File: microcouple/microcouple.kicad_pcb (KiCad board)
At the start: 4 copper layers, 29.3 x 37.5 mm, 127 parts, among them J1 Conn_ARM_SWD_TagConnect_TC203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, P1 USB_C_Plug, Q1 AO3415, SW1 ~{RESET}, SW2 SW_SPDT_MSK12CO2, SW3 CS2, SW4 CS3, SW5 CS4, U1 USBLC6-2SC6, U2 RP2040, U3 MCP73831-2-OT, U4 LM3671MFX, U5 IRM-V838M3-C/TR1, U6 IS31FL3729, U7 CAP1188, X1 12MHz 12pF

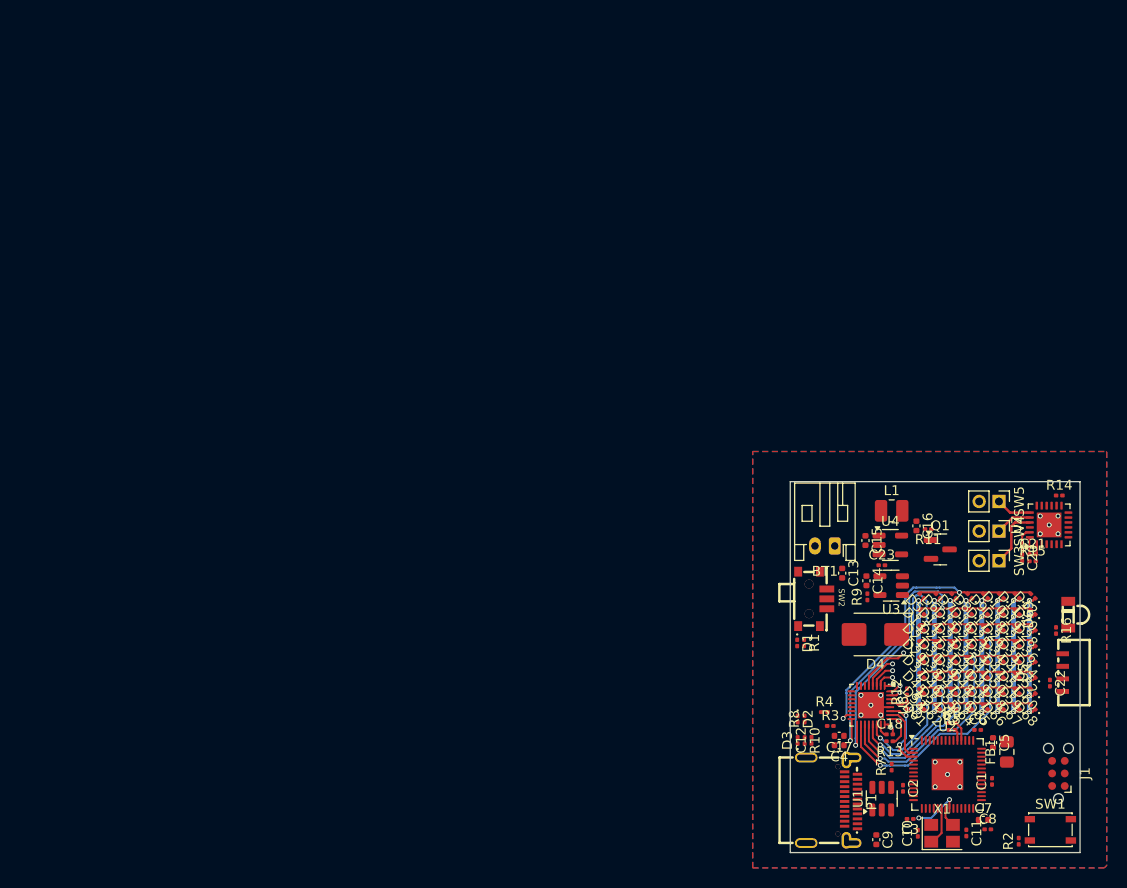
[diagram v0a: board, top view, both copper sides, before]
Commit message: Draft layout
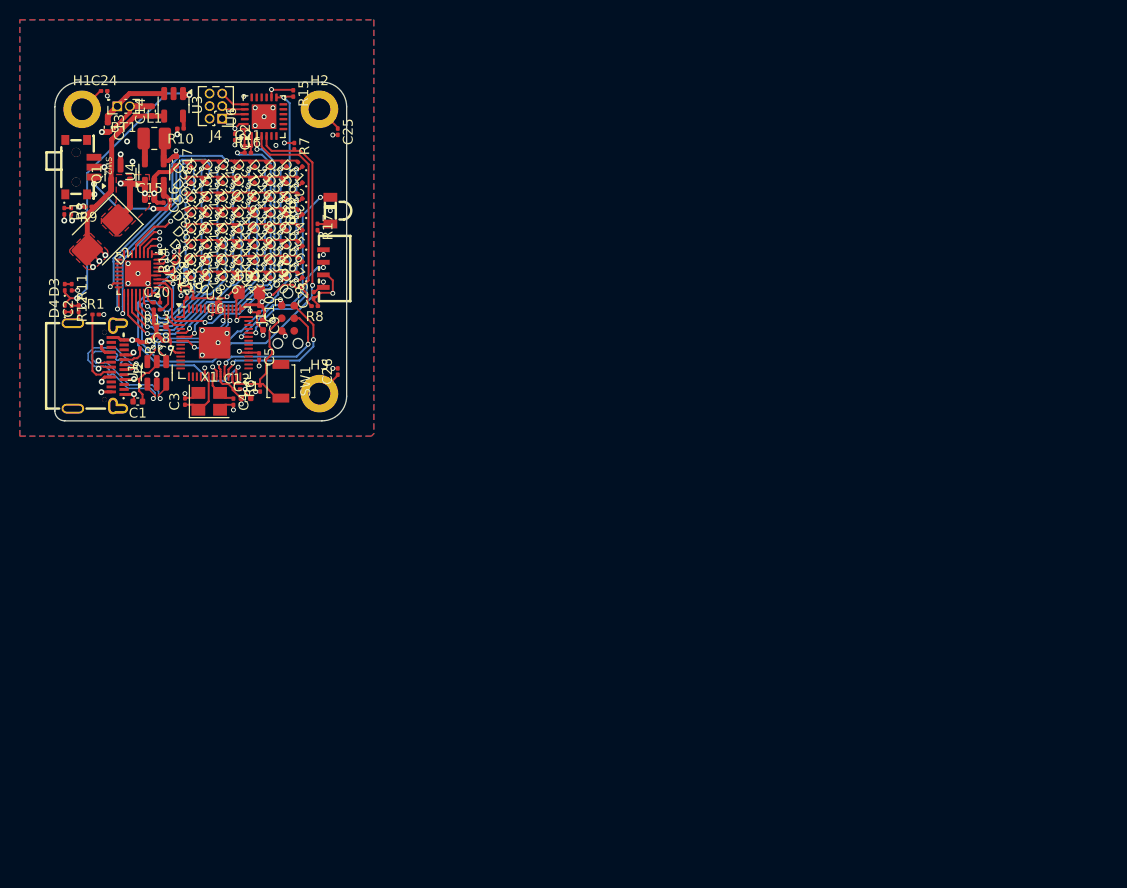
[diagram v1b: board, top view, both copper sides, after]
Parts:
- removed the C17 at (165.4, 110.7)
- removed the C9 at (169.2, 121.2)
- removed R5: 27R, Resistor_SMD:R_0201_0603Metric
- removed the R6 at (176.8, 109.4)
- removed SW3: CS2, Connector_PinHeader_2.00mm:PinHeader_1x02_P2.00mm_Vertical
- removed SW4: CS3, Connector_PinHeader_2.00mm:PinHeader_1x02_P2.00mm_Vertical
- removed SW5: CS4, Connector_PinHeader_2.00mm:PinHeader_1x02_P2.00mm_Vertical
- added C1: 4.7uF, Capacitor_SMD:C_0402_1005Metric, F.Cu at (94.5, 76.9)
- added C19: 100nF, Capacitor_SMD:C_0201_0603Metric, F.Cu at (99.8, 66.5)
- added C24: 100nF, Capacitor_SMD:C_0201_0603Metric, F.Cu at (91.1, 45.5)
- added C25: 100nF, Capacitor_SMD:C_0201_0603Metric, F.Cu at (114.8, 49.6)
- added C26: 100nF, Capacitor_SMD:C_0201_0603Metric, F.Cu at (114.8, 73.9)
- added H1: MountingHole_Pad, MountingHole:MountingHole_2.2mm_M2_DIN965_Pad, F.Cu at (88.9, 47.4)
- added H2: MountingHole_Pad, MountingHole:MountingHole_2.2mm_M2_DIN965_Pad, F.Cu at (112.9, 47.4)
- added H3: MountingHole_Pad, MountingHole:MountingHole_2.2mm_M2_DIN965_Pad, F.Cu at (112.9, 76.1)
- added J4: Conn_02x03_Odd_Even, Connector_PinHeader_1.27mm:PinHeader_2x03_P1.27mm_Vertical, F.Cu at (103.1, 48.3)
- added R2: 5.1k, Resistor_SMD:R_0201_0603Metric, F.Cu at (94.8, 71.2)
- BT1: footprint Connector_JST:JST_PH_S2B-PH-K_1x02_P2.00mm_Horizontal -> Connector_PinSocket_1.27mm:PinSocket_2x01_P1.27mm_Vertical
- J2: renamed from P1; value USB_C_Plug -> USB_C_Socket
- SW1: footprint Button_Switch_SMD:SW_SPST_PTS810 -> Button_Switch_SMD:SW_SPST_B3U-1000P
- moved R1 92.6 mm to (90.3, 68.1), turned to 0 degrees
- moved Q1 91.1 mm to (92.8, 54.0), turned to 90 degrees
- moved R9 90.9 mm to (89.5, 57.2)
- moved J1 90.5 mm to (109.7, 68.5), turned to -90 degrees
- moved C22 90.3 mm to (104.3, 50.1)
- moved SW1 90.1 mm to (109.0, 74.8), turned to -90 degrees
- moved FB1 89.6 mm to (105.8, 65.8), turned to 0 degrees
- moved U6 89.5 mm to (107.3, 48.1)
- moved R16 89.5 mm to (105.7, 51.8)
- moved C21 89.5 mm to (105.7, 51.0)
- moved C7 89.4 mm to (97.4, 70.8)
- moved R6 89.3 mm to (106.9, 75.6)
- moved C12 88.0 mm to (104.5, 75.7)
- moved D2 88.0 mm to (91.0, 60.0), turned to -135 degrees
- moved R15 87.5 mm to (110.2, 45.8), turned to -90 degrees
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- renumbered C6 to C10, C7 to C11, C8 to C12, C23 to C16, C16 to C17, C19 to C18, C12 to C2, C18 to C20, C20 to C22, C22 to C23, C10 to C3, C11 to C4, C1 to C5, C2 to C6, C3 to C7, C4 to C8, C5 to C9, D45 to D10, D53 to D11, D61 to D12, D6 to D13, D22 to D15, D30 to D16, D38 to D17, D46 to D18, D54 to D19, D4 to D2, D62 to D20, D7 to D21, D15 to D22, D31 to D24, D39 to D25, D47 to D26, D55 to D27, D63 to D28, D8 to D29, D2 to D3, D16 to D30, D24 to D31, D40 to D33, D48 to D34, D56 to D35, D64 to D36, D9 to D37, D17 to D38, D25 to D39, D3 to D4, D33 to D40, D49 to D42, D57 to D43, D65 to D44, D10 to D45, D18 to D46, D26 to D47, D34 to D48, D42 to D49, D58 to D51, D66 to D52, D11 to D53, D19 to D54, D27 to D55, D35 to D56, D43 to D57, D51 to D58, D13 to D6, D67 to D60, D12 to D61, D20 to D62, D28 to D63, D36 to D64, D44 to D65, D52 to D66, D60 to D67, D21 to D7, D29 to D8, D37 to D9, R7 to R1, R9 to R10, R8 to R11, R10 to R12, R12 to R14, R14 to R15, R15 to R16, R16 to R17, R1 to R3, R2 to R6, R3 to R7, R4 to R8, R11 to R9, U6 to U5, U7 to U6, U5 to U7
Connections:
- J2 pad A5: Net-(P1-CC) -> Net-(J2-CC1)
- J2 pad B5: unconnected-(P1-VCONN-PadB5) -> Net-(J2-CC2)
- R1 pad 1: Net-(P1-CC) -> Net-(J2-CC2)
- U2 pad 46: Net-(U2-USB_DM) -> /USB.D_PROTECTED-
- U2 pad 47: Net-(U2-USB_DP) -> /USB.D_PROTECTED+
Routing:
- net GND: track 5.13 -> 58.2 mm, vias 17 -> 51
- net /I2C0.SDL: track 7.20 -> 54.9 mm, vias 2 -> 3
- net VBUS: track 0.00 -> 36.1 mm, vias 0 -> 8
- net /I2C0.SDA: track 5.55 -> 41.2 mm, vias 0 -> 2
- net /~{CT_ALERT}: track 0.00 -> 34.8 mm, vias 0 -> 2
- net /Battery Management/Charge Status: track 0.00 -> 30.2 mm, vias 0 -> 2
- net +3.3V: track 8.94 -> 37.6 mm, vias 2 -> 14
- net /CT_RESET: track 1.74 -> 30.4 mm, vias 0 -> 2
- net /CT_WAKE: track 0.00 -> 28.2 mm, vias 0 -> 2
- net /~{MX_SDB}: track 2.61 -> 29.9 mm, vias 0 -> 2
- net /IR.TX: track 0.00 -> 21.2 mm, vias 0 -> 2
- net /USB.D+: track 0.00 -> 20.7 mm, vias 0 -> 3
- net /USB.D-: track 0.00 -> 20.7 mm, vias 0 -> 3
- net Net-(J2-SHIELD): track 0.00 -> 18.9 mm
- net /SWDIO: track 0.00 -> 15.3 mm, vias 0 -> 2
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- added copper zone on F.Cu, net +3.3V
- added copper zone on In2.Cu, net +3.3V
- added copper zone on F.Cu, net /Battery Management/VIN
- added copper zone on F.Cu, net VBUS
- added copper zone on In2.Cu, net VBUS
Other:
- board size 29.3 x 37.5 mm -> 29.5 x 34.2 mm
